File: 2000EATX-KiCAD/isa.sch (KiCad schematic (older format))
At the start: 6 parts, among them CN1 Bus_ISA_8bit, CN2 Bus_ISA_16bit, CN3 Bus_ISA_8bit, CN4 Bus_ISA_16bit, CN5 Bus_ISA_16bit, CN6 Bus_ISA_8bit

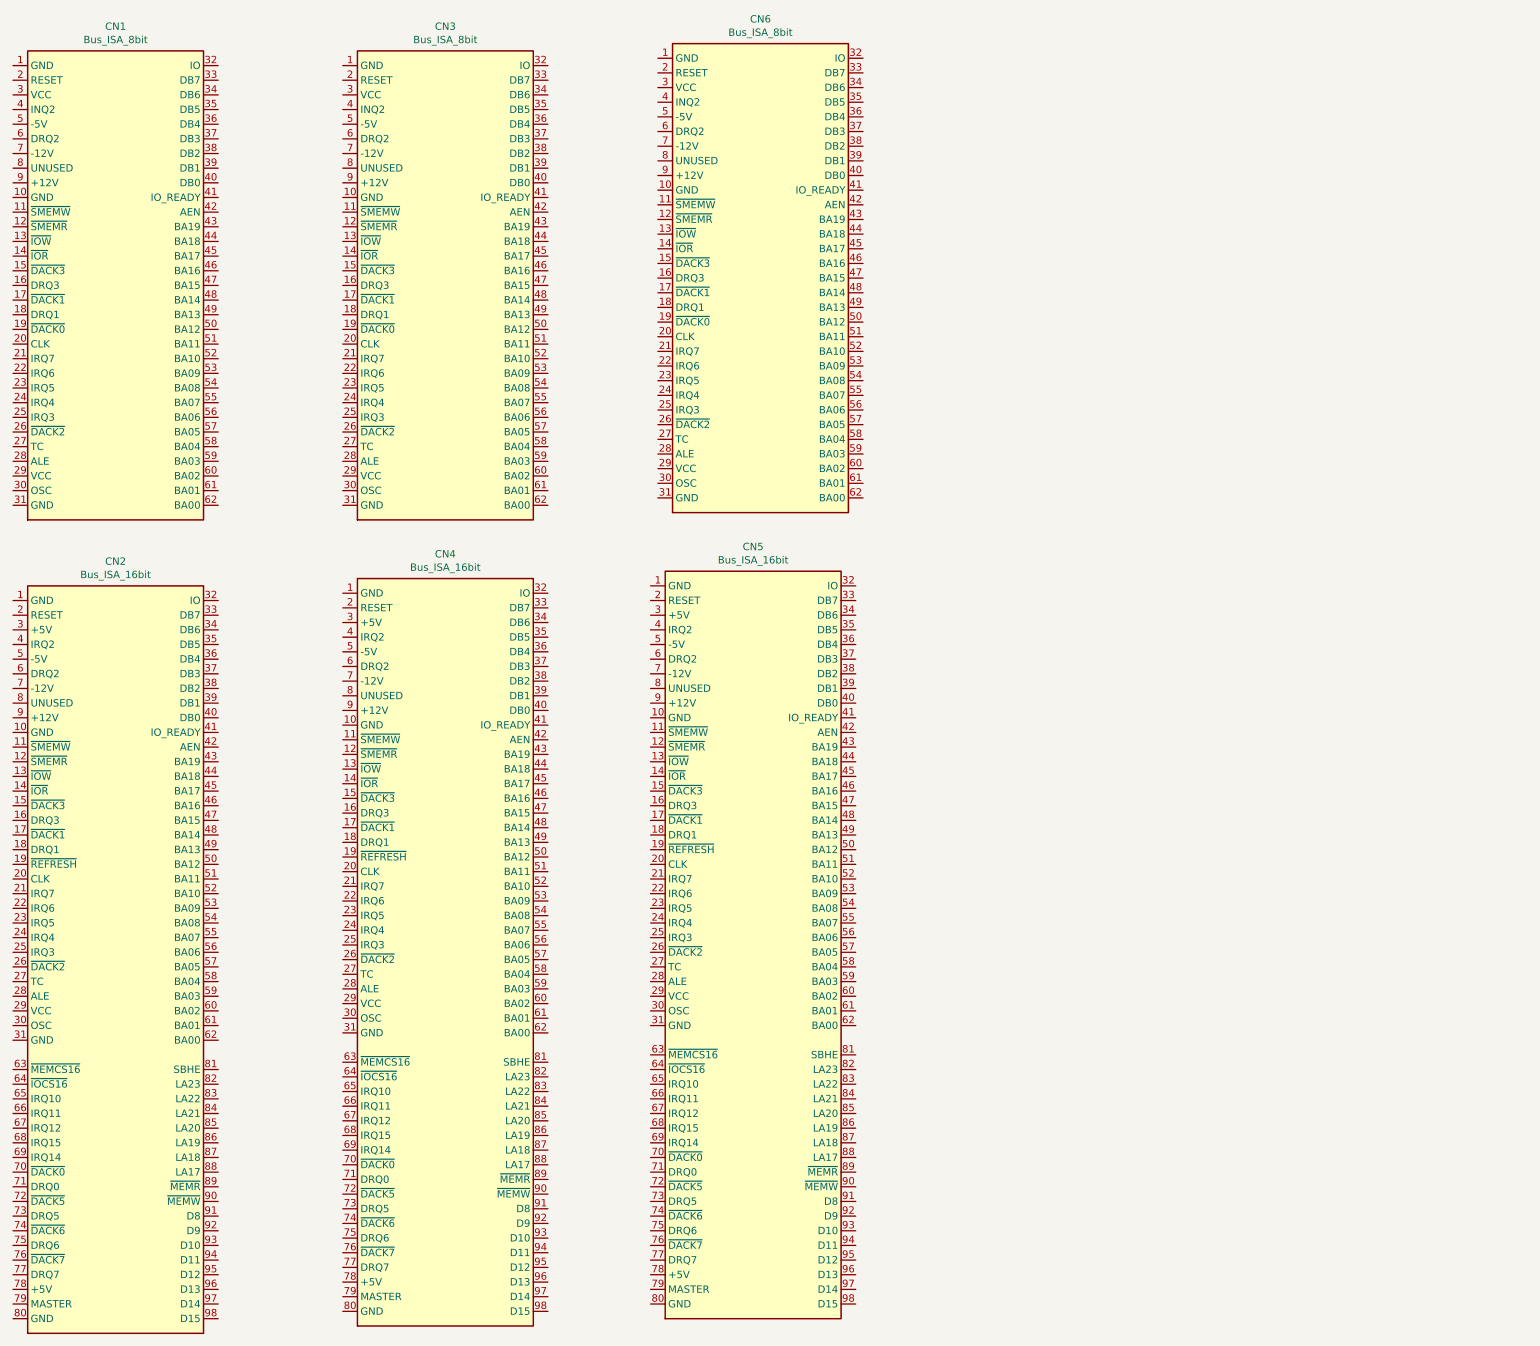
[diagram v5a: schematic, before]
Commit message: Add files via upload
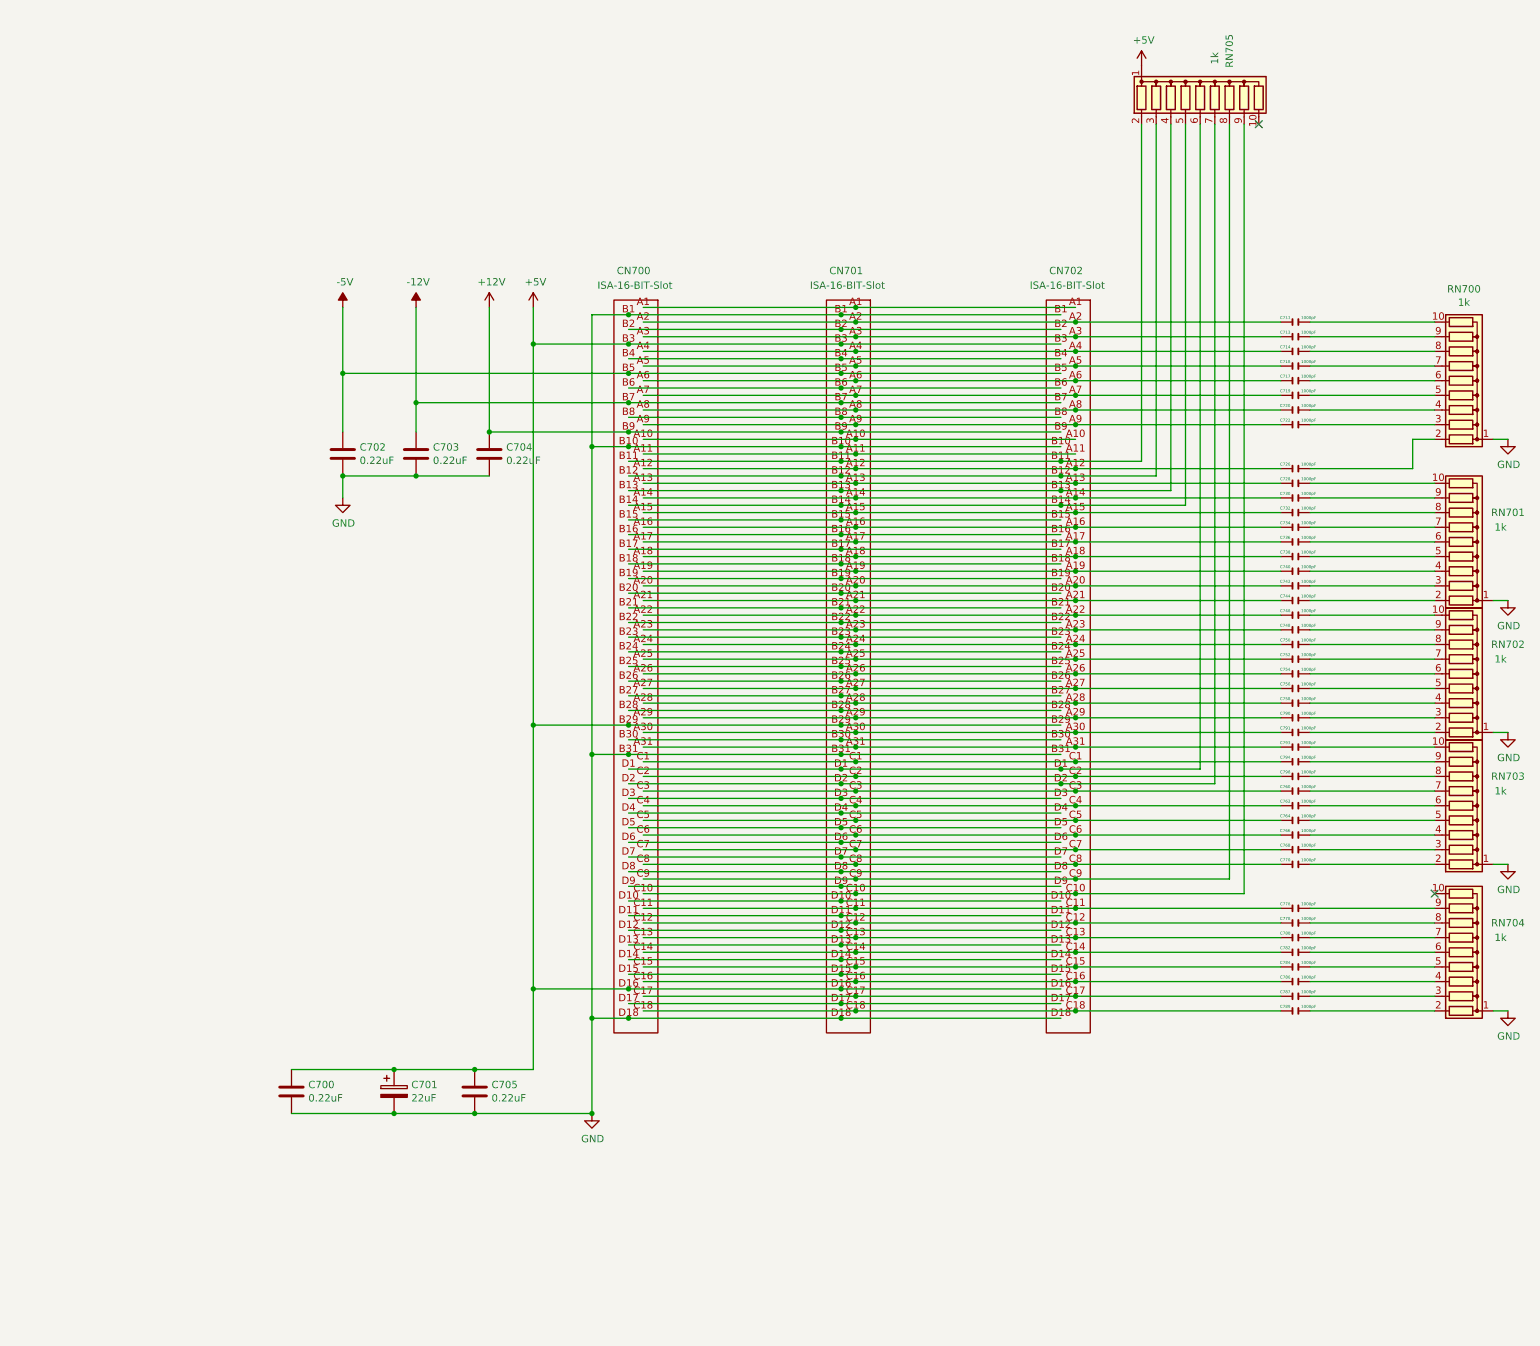
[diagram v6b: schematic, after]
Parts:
- removed CN1, CN3, CN6: Bus_ISA_8bit, AmigaFootprints:ISA_2x31_P2.54mm_Horizontal, symbol Connector:Bus_ISA_8bit
- removed CN2, CN4, CN5: Bus_ISA_16bit, Connector_Samtec_HLE_THT:Samtec_HLE-118-02-xx-DV-TE_2x18_P2.54mm_Horizontal, symbol Connector:Bus_ISA_16bit
- added C700, C702, C703, C704, C705: 0.22uF, Capacitor_SMD:C_1206_3216Metric, symbol Device:C
- added C701: 22uF, Capacitor_SMD:CP_Elec_6.3x5.8, symbol Device:CP
- added C711, C713, C714, C716, C717, C719, C720, C722, C726, C728, C730, C732, C734, C736, C738, C740, C742, C744, C746, C748, C750, C752, C754, C756, C758, C760, C762, C764, C766, C768, C770, C776, C778, C780, C782, C784, C786, C787, C789, C790, C791, C793, C794, C796: 1000pF, Capacitor_SMD:C_1206_3216Metric, symbol Amiga-Library:C_Small
- added CN700, CN701, CN702: ISA-16-BIT-Slot, AmigaFootprints:ISA_16-BIT_P2.54mm_Horizontal, symbol Amiga-Library:ISA-16-BIT-Slot
- added RN700, RN701, RN702, RN703, RN704, RN705: 1k, Resistor_THT:R_Array_SIP10, symbol Device:R_Network09
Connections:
- new net: C711.1, RN700.10 (R9)
- new net: C711.2, CN700.A2, CN701.A2, CN702.A2
- new net: C713.1, RN700.9 (R8)
- new net: C713.2, CN700.A3, CN701.A3, CN702.A3
- new net: C714.1, RN700.8 (R7)
- new net: C714.2, CN700.A4, CN701.A4, CN702.A4
- new net: C716.1, RN700.7 (R6)
- new net: C716.2, CN700.A5, CN701.A5, CN702.A5
- new net: C717.1, RN700.6 (R5)
- new net: C717.2, CN700.A6, CN701.A6, CN702.A6
- new net: C719.1, RN700.5 (R4)
- new net: C719.2, CN700.A7, CN701.A7, CN702.A7
- new net: C720.1, RN700.4 (R3)
- new net: C720.2, CN700.A8, CN701.A8, CN702.A8
- new net: C722.1, RN700.3 (R2)
- new net: C722.2, CN700.A9, CN701.A9, CN702.A9
- new net: C726.1, RN700.2 (R1)
- new net: C726.2, CN700.A12, CN701.A12, CN702.A12
- new net: C728.1, RN701.10 (R9)
- new net: C728.2, CN700.A13, CN701.A13, CN702.A13
- new net: C730.1, RN701.9 (R8)
- new net: C730.2, CN700.A14, CN701.A14, CN702.A14
- new net: C732.1, RN701.8 (R7)
- new net: C732.2, CN700.A15, CN701.A15, CN702.A15
- new net: C734.1, RN701.7 (R6)
- new net: C734.2, CN700.A16, CN701.A16, CN702.A16
- new net: C736.1, RN701.6 (R5)
- new net: C736.2, CN700.A17, CN701.A17, CN702.A17
- new net: C738.1, RN701.5 (R4)
- new net: C738.2, CN700.A18, CN701.A18, CN702.A18
- new net: C740.1, RN701.4 (R3)
- new net: C740.2, CN700.A19, CN701.A19, CN702.A19
- new net: C742.1, RN701.3 (R2)
- new net: C742.2, CN700.A20, CN701.A20, CN702.A20
- new net: C744.1, RN701.2 (R1)
- new net: C744.2, CN700.A21, CN701.A21, CN702.A21
- new net: C746.1, RN702.10 (R9)
- new net: C746.2, CN700.A22, CN701.A22, CN702.A22
- new net: C748.1, RN702.9 (R8)
- new net: C748.2, CN700.A23, CN701.A23, CN702.A23
- new net: C750.1, RN702.8 (R7)
- new net: C750.2, CN700.A24, CN701.A24, CN702.A24
- new net: C752.1, RN702.7 (R6)
- new net: C752.2, CN700.A25, CN701.A25, CN702.A25
- new net: C754.1, RN702.6 (R5)
- new net: C754.2, CN700.A26, CN701.A26, CN702.A26
- new net: C756.1, RN702.5 (R4)
- new net: C756.2, CN700.A27, CN701.A27, CN702.A27
- new net: C758.1, RN702.4 (R3)
- new net: C758.2, CN700.A28, CN701.A28, CN702.A28
- new net: C790.1, RN702.3 (R2)
- new net: C790.2, CN700.A29, CN701.A29, CN702.A29
- new net: C791.1, RN702.2 (R1)
- new net: C791.2, CN700.A30, CN701.A30, CN702.A30
- new net: C793.1, RN703.10 (R9)
- new net: C793.2, CN700.A31, CN701.A31, CN702.A31
- new net: C794.1, RN703.9 (R8)
- new net: C794.2, CN700.C1, CN701.C1, CN702.C1
- new net: C796.1, RN703.8 (R7)
- new net: C796.2, CN700.C2, CN701.C2, CN702.C2
- new net: C760.1, RN703.7 (R6)
- new net: C760.2, CN700.C3, CN701.C3, CN702.C3
- new net: C762.1, RN703.6 (R5)
- new net: C762.2, CN700.C4, CN701.C4, CN702.C4
- new net: C764.1, RN703.5 (R4)
- new net: C764.2, CN700.C5, CN701.C5, CN702.C5
- new net: C766.1, RN703.4 (R3)
- new net: C766.2, CN700.C6, CN701.C6, CN702.C6
- new net: C768.1, RN703.3 (R2)
- new net: C768.2, CN700.C7, CN701.C7, CN702.C7
- new net: C770.1, RN703.2 (R1)
- new net: C770.2, CN700.C8, CN701.C8, CN702.C8
- new net: C789.1, RN704.2 (R1)
- new net: C789.2, CN700.C18, CN701.C18, CN702.C18
- new net: C787.1, RN704.3 (R2)
- new net: C787.2, CN700.C17, CN701.C17, CN702.C17
- new net: C786.1, RN704.4 (R3)
- new net: C786.2, CN700.C16, CN701.C16, CN702.C16
- new net: C784.1, RN704.5 (R4)
- new net: C784.2, CN700.C15, CN701.C15, CN702.C15
- new net: C782.1, RN704.6 (R5)
- new net: C782.2, CN700.C14, CN701.C14, CN702.C14
- new net: C780.1, RN704.7 (R6)
- new net: C780.2, CN700.C13, CN701.C13, CN702.C13
- new net: C778.1, RN704.8 (R7)
- new net: C778.2, CN700.C12, CN701.C12, CN702.C12
- new net: C776.1, RN704.9 (R8)
- new net: C776.2, CN700.C11, CN701.C11, CN702.C11
- new net: CN700.B11, CN701.B11, CN702.B11, RN705.2 (R1)
- new net: CN700.B12, CN701.B12, CN702.B12, RN705.3 (R2)
- new net: CN700.B13, CN701.B13, CN702.B13, RN705.4 (R3)
- new net: CN700.B14, CN701.B14, CN702.B14, RN705.5 (R4)
- new net: CN700.D1, CN701.D1, CN702.D1, RN705.6 (R5)
- new net: CN700.D2, CN701.D2, CN702.D2, RN705.7 (R6)
- new net: CN700.C9, CN701.C9, CN702.C9, RN705.8 (R7)
- new net: CN700.C10, CN701.C10, CN702.C10, RN705.9 (R8)
- new net: CN700.A1, CN701.A1, CN702.A1
- new net: CN700.A10, CN701.A10, CN702.A10
- new net: CN700.A11, CN701.A11, CN702.A11
- new net: CN700.B15, CN701.B15, CN702.B15
- new net: CN700.B16, CN701.B16, CN702.B16
- new net: CN700.B17, CN701.B17, CN702.B17
- new net: CN700.B18, CN701.B18, CN702.B18
- new net: CN700.B19, CN701.B19, CN702.B19
- new net: CN700.B2, CN701.B2, CN702.B2
- new net: CN700.B20, CN701.B20, CN702.B20
- new net: CN700.B21, CN701.B21, CN702.B21
- new net: CN700.B22, CN701.B22, CN702.B22
- new net: CN700.B23, CN701.B23, CN702.B23
- new net: CN700.B24, CN701.B24, CN702.B24
- new net: CN700.B25, CN701.B25, CN702.B25
- new net: CN700.B26, CN701.B26, CN702.B26
- new net: CN700.B27, CN701.B27, CN702.B27
- new net: CN700.B28, CN701.B28, CN702.B28
- new net: CN700.B30, CN701.B30, CN702.B30
- new net: CN700.B4, CN701.B4, CN702.B4
- new net: CN700.B6, CN701.B6, CN702.B6
- new net: CN700.B8, CN701.B8, CN702.B8
- new net: CN700.D10, CN701.D10, CN702.D10
- new net: CN700.D11, CN701.D11, CN702.D11
- new net: CN700.D12, CN701.D12, CN702.D12
- new net: CN700.D13, CN701.D13, CN702.D13
- new net: CN700.D14, CN701.D14, CN702.D14
- new net: CN700.D15, CN701.D15, CN702.D15
- new net: CN700.D17, CN701.D17, CN702.D17
- new net: CN700.D3, CN701.D3, CN702.D3
- new net: CN700.D4, CN701.D4, CN702.D4
- new net: CN700.D5, CN701.D5, CN702.D5
- new net: CN700.D6, CN701.D6, CN702.D6
- new net: CN700.D7, CN701.D7, CN702.D7
- new net: CN700.D8, CN701.D8, CN702.D8
- new net: CN700.D9, CN701.D9, CN702.D9
- new net +12V: C704.1, CN700.B9, CN701.B9, CN702.B9
- new net +5V: C700.1, C701.1, C705.1, CN700.B29, CN700.B3, CN700.D16, CN701.B29, CN701.B3, CN701.D16, CN702.B29, CN702.B3, CN702.D16, RN705.1 (common)
- new net -12V: C703.1, CN700.B7, CN701.B7, CN702.B7
- new net -5V: C702.1, CN700.B5, CN701.B5, CN702.B5
- new net GND: C700.2, C701.2, C702.2, C703.2, C704.2, C705.2, CN700.B1, CN700.B10, CN700.B31, CN700.D18, CN701.B1, CN701.B10, CN701.B31, CN701.D18, CN702.B1, CN702.B10, CN702.B31, CN702.D18, RN700.1 (common), RN701.1 (common), RN702.1 (common), RN703.1 (common), RN704.1 (common)
- no-connect marks 0 -> 2
